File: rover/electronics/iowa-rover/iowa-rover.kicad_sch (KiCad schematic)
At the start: 10 parts, among them J1 Adafruit_USB_C, J2 Conn_01x02, J3 Conn_01x02, U1 Adafruit_Metro_Mini, U2 Adafruit_RFM69HCW_Breakout, U3 Adafruit_TB6612_Breakout

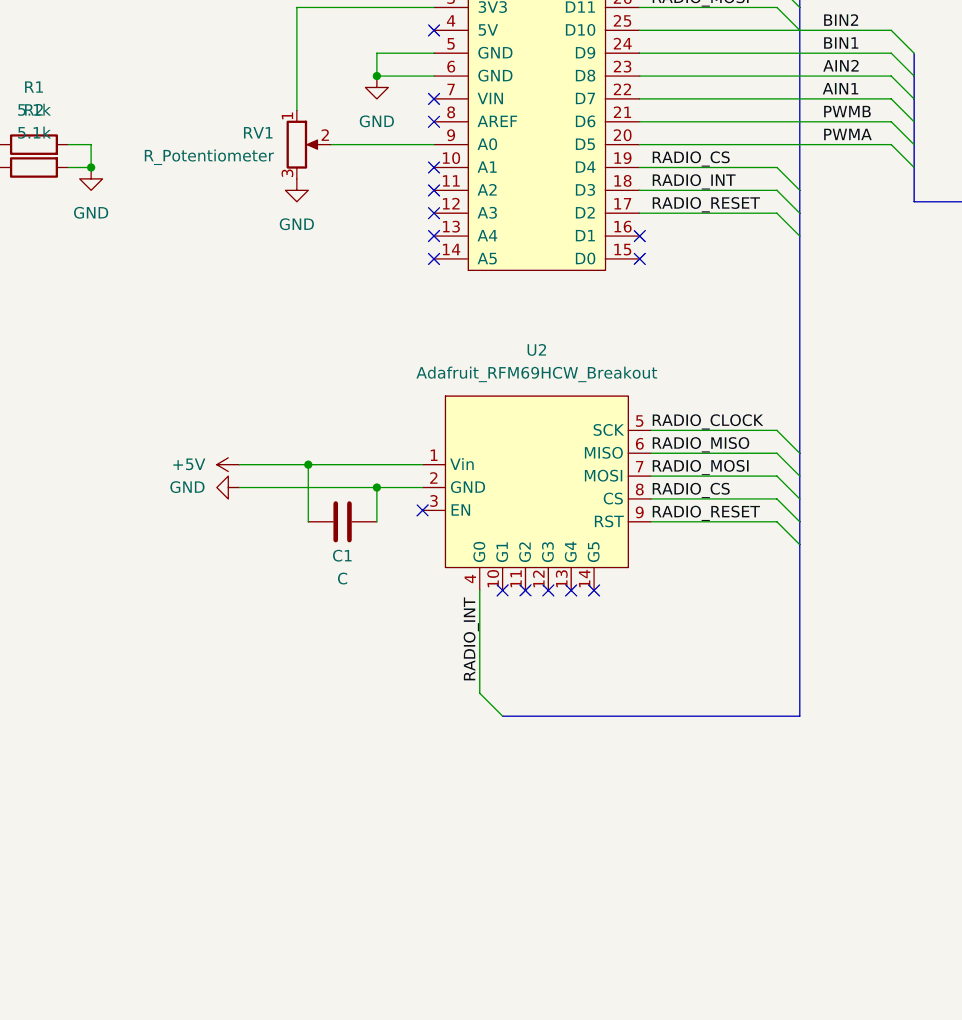
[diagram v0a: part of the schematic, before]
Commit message: update
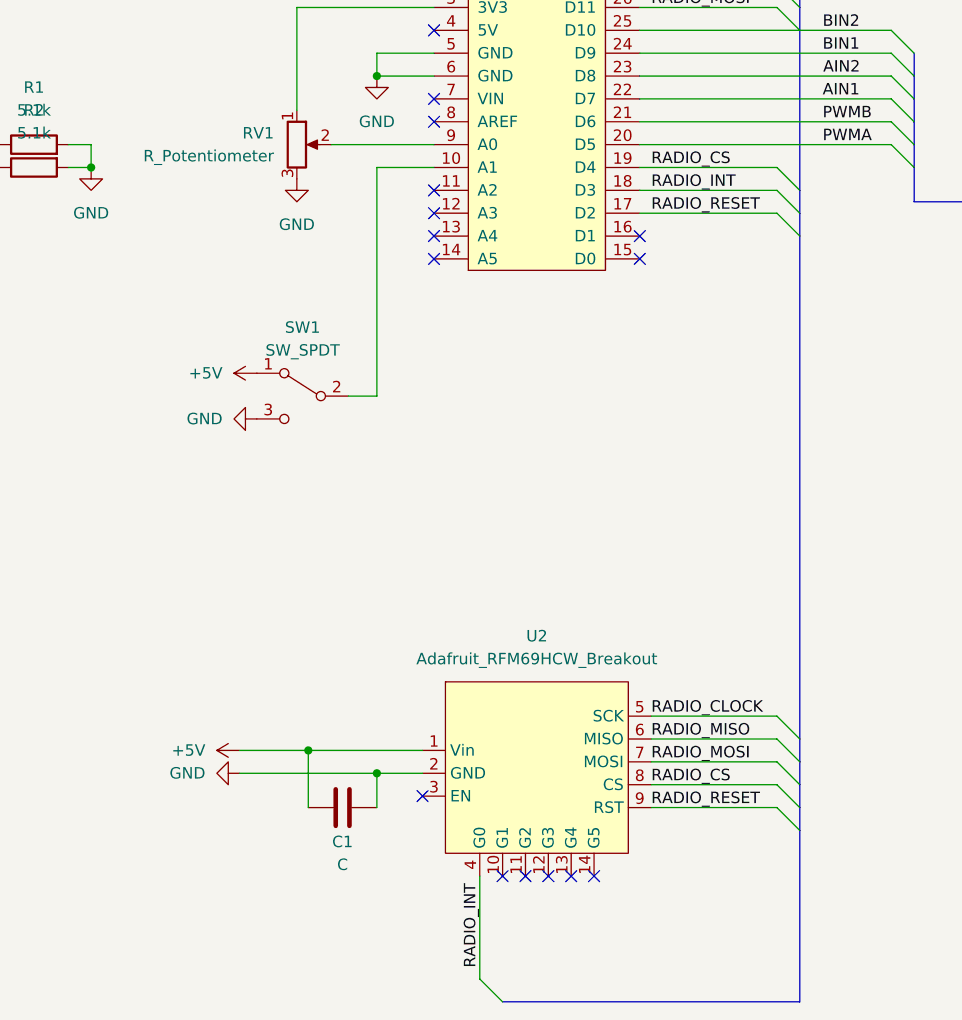
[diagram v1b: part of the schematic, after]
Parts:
- added SW1: SW_SPDT, SMM:SW_EG1218, symbol Switch:SW_SPDT
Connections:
- net +5V: now also SW1.1 (A)
- net GND: now also SW1.3 (C)
- net at U1.10 (A1): now also SW1.2 (B)
- no-connect marks 18 -> 17
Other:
- moved on the sheet: C1, U2
